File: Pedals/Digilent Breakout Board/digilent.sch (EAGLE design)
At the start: 5 parts

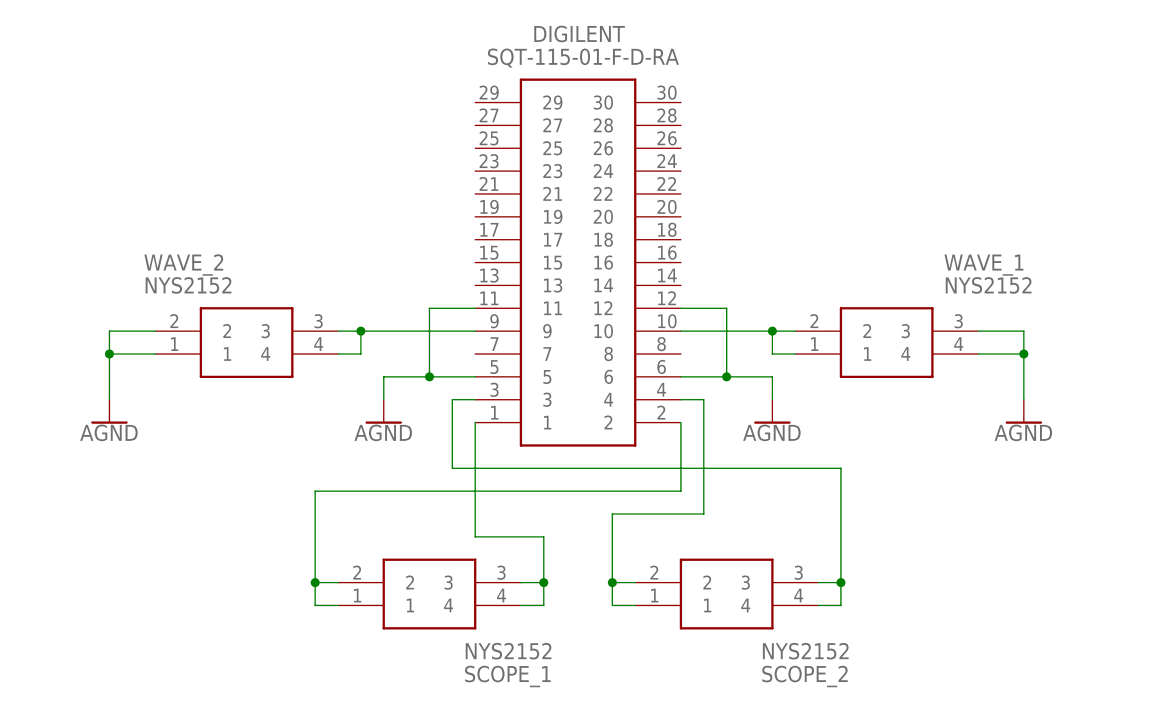
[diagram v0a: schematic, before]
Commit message: Route board
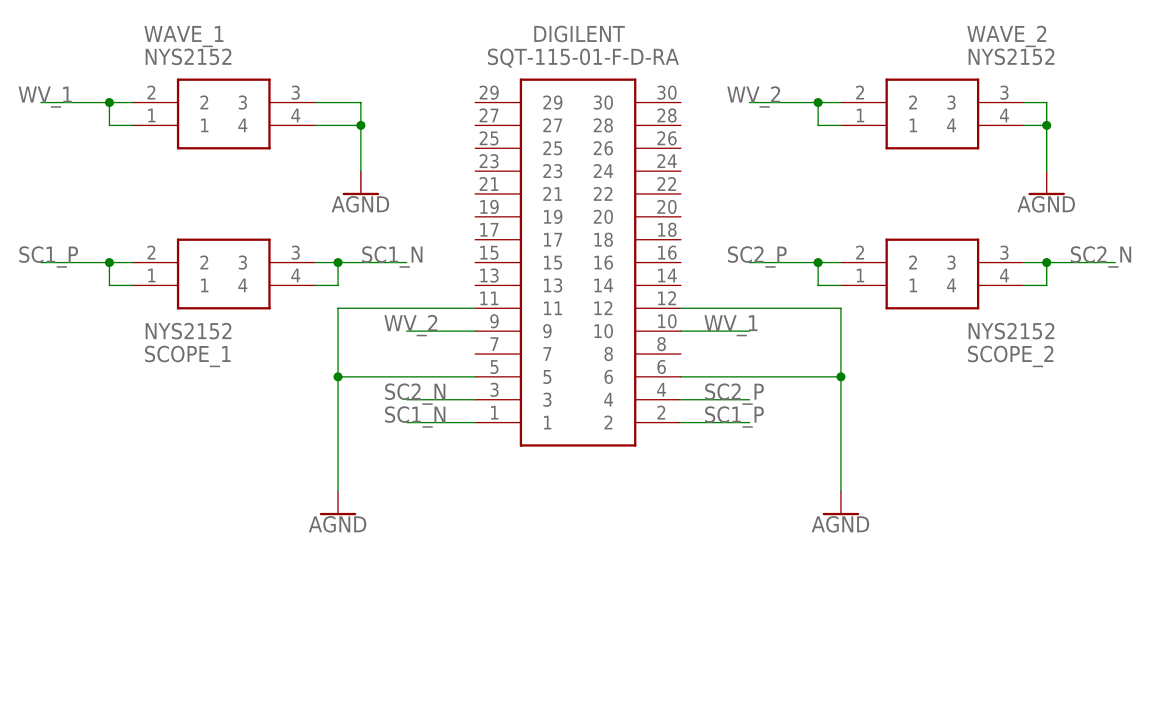
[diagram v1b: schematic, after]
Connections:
- net N$1 renamed SC1_P
- net N$2 renamed SC2_P
- net N$3 renamed SC1_N
- net N$4 renamed SC2_N
- net N$7 renamed WV_1
- removed net N$5: DIGILENT.9, WAVE_2.3, WAVE_2.4
- new net WV_2: DIGILENT.9, WAVE_2.1, WAVE_2.2
- net AGND: now also WAVE_2.3, WAVE_2.4; no longer WAVE_2.1, WAVE_2.2
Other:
- moved on the sheet: SCOPE_1, SCOPE_2, WAVE_1, WAVE_2
